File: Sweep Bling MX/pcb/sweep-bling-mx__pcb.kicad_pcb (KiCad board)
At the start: 2 copper layers, 113.5 x 95.2 mm, 31 parts, among them J2 AudioJack4dpb, SW10 SW_Push, SW11 SW_Push, SW12 SW_Push, SW14 SW_Push, SW15 SW_Push, SW16 SW_Push, SW17 SW_Push, SW18 SW_Push, SW2 SW_Push, SW20 SW_Push, SW21 SW_Push, SW3 SW_Push, SW4 SW_Push, SW5 SW_Push, SW6 SW_Push, SW8 SW_Push, SW9 SW_Push, U1 ProMicro-kbd

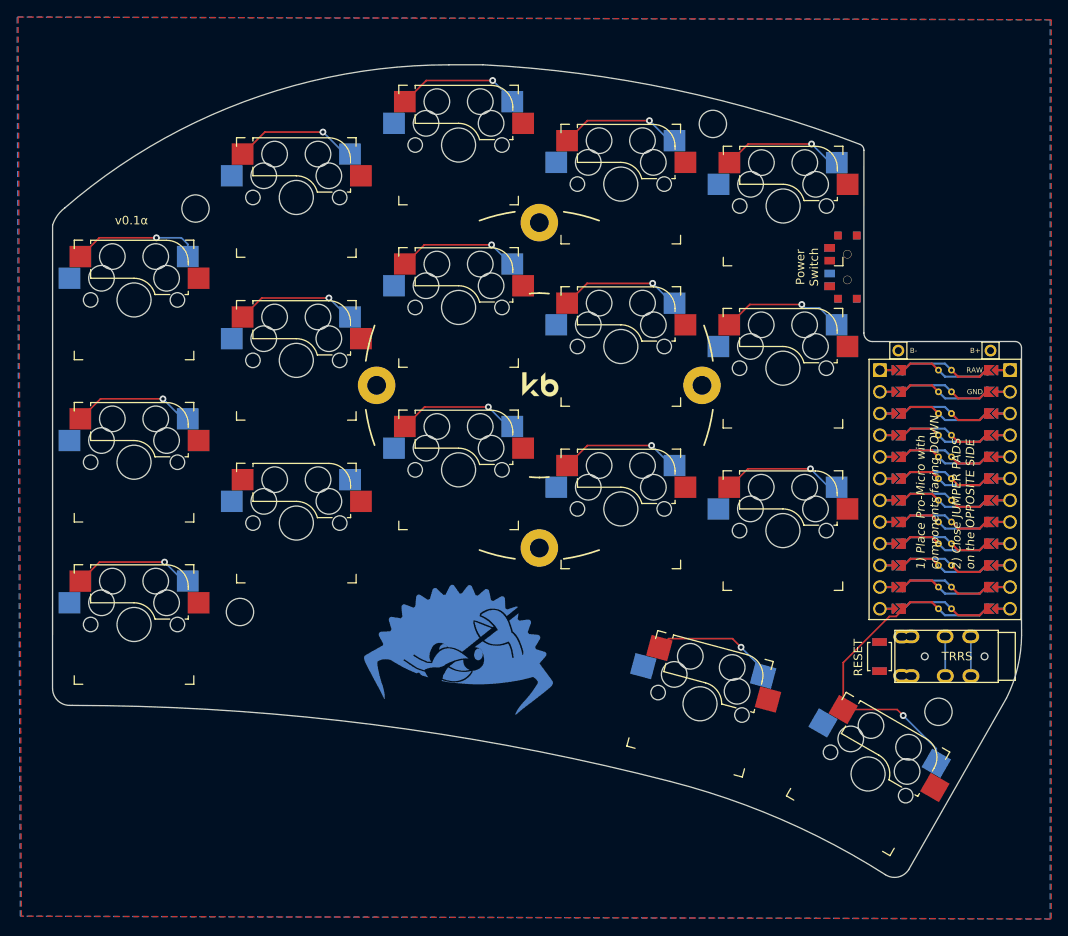
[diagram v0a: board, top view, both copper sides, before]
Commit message: Finish manual routing
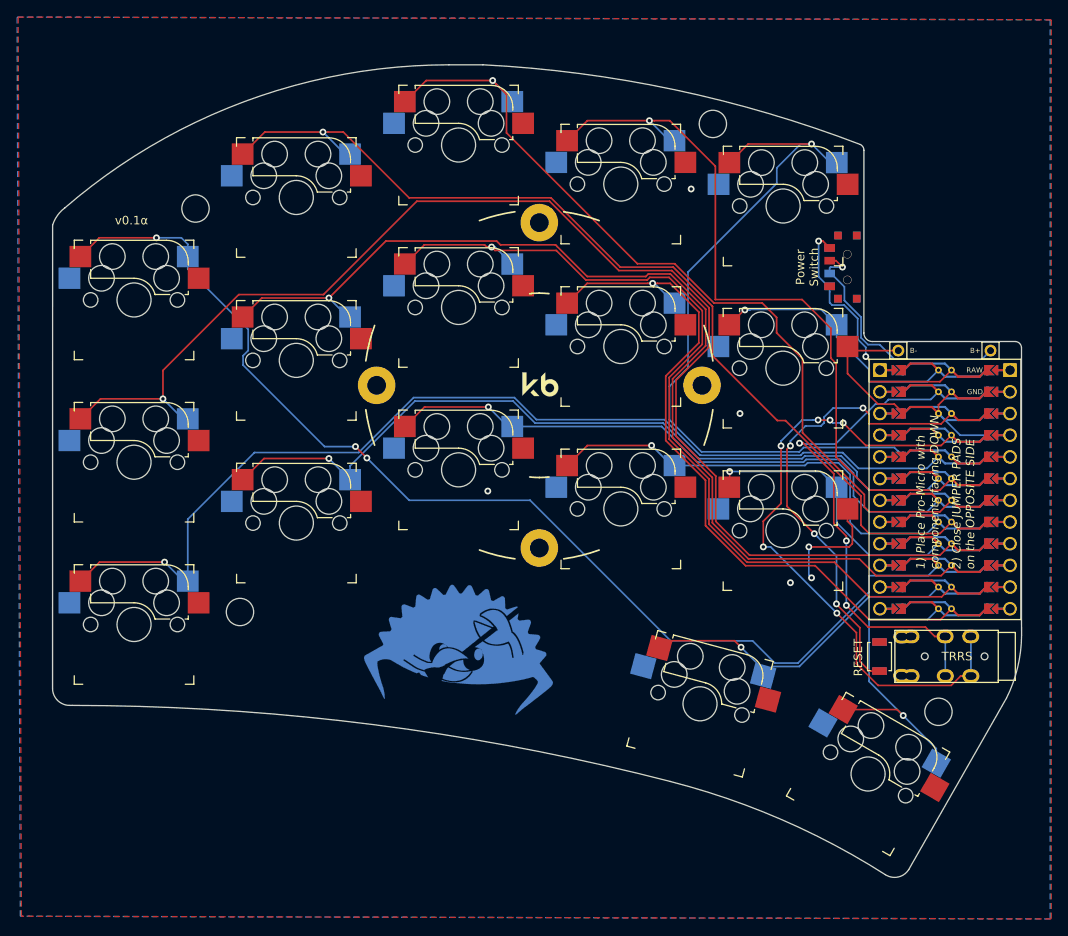
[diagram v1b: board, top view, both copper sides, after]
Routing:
- net Switch6: track 14.5 -> 153.5 mm
- net Switch1: track 15.2 -> 132.9 mm, vias 1 -> 3
- net Switch7: track 14.4 -> 124.5 mm
- net Switch11: track 14.4 -> 119.7 mm
- net Switch2: track 14.7 -> 113.7 mm
- net Switch12: track 0.00 -> 93.8 mm, vias 0 -> 1
- net Switch8: track 14.4 -> 103.4 mm
- net Switch3: track 14.7 -> 99.6 mm
- net Switch4: track 14.5 -> 86.0 mm
- net Switch5: track 14.4 -> 84.0 mm
- net vcc: track 4.64 -> 74.2 mm, vias 0 -> 6
- net Switch9: track 14.5 -> 83.7 mm
- net Switch13: track 14.5 -> 70.9 mm
- net reset: track 0.00 -> 55.1 mm, vias 0 -> 4
- net Switch18: track 4.64 -> 58.1 mm, vias 0 -> 3
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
